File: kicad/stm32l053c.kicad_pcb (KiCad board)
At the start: 2 copper layers, 52 x 35 mm, 39 parts, among them P1 SWD, P2 PWR, Q1 BC807, Q2 BC817, SW1 SW_PUSH, SW2 SW_PUSH, SW3 SW_PUSH, SW4 SW_SPDT, U1 STM32L053C8_LQFP48, U2 TLV61225, U3 um66t, Y1 Crystal_GND23

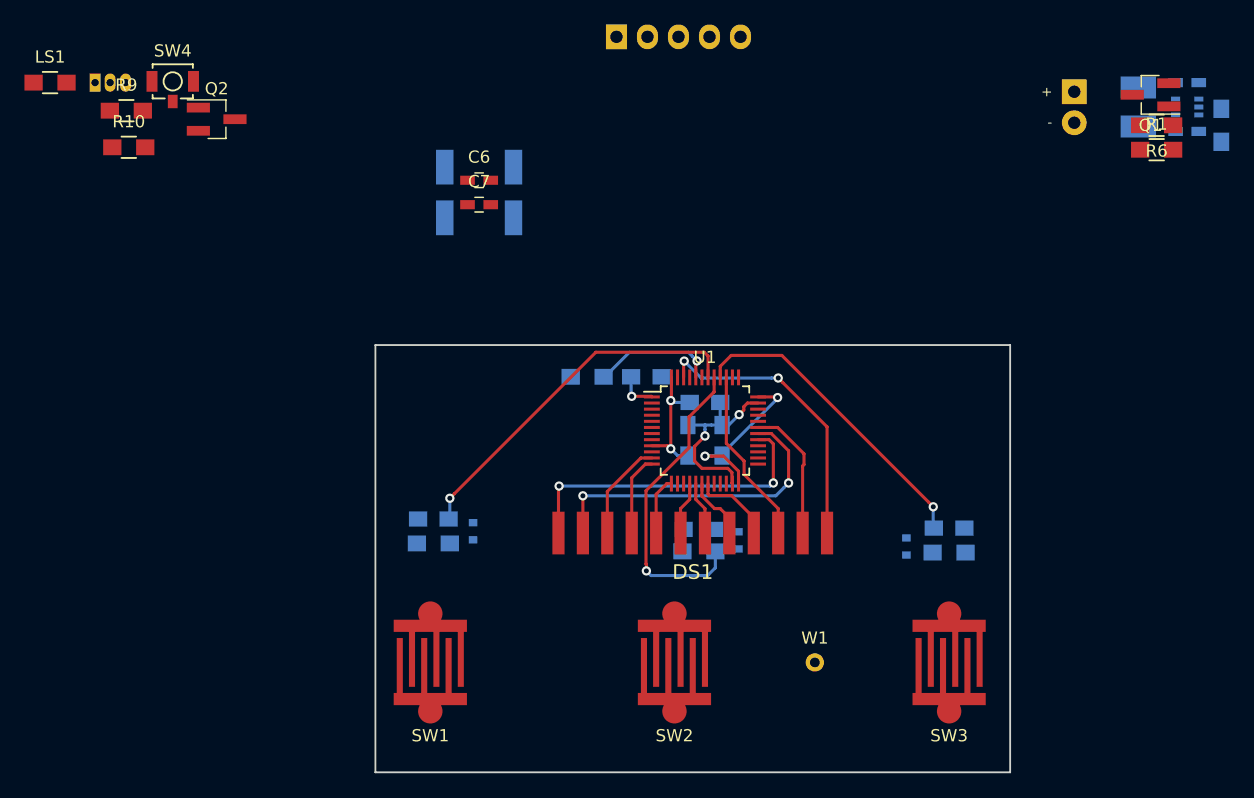
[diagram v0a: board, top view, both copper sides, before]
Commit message: Layout
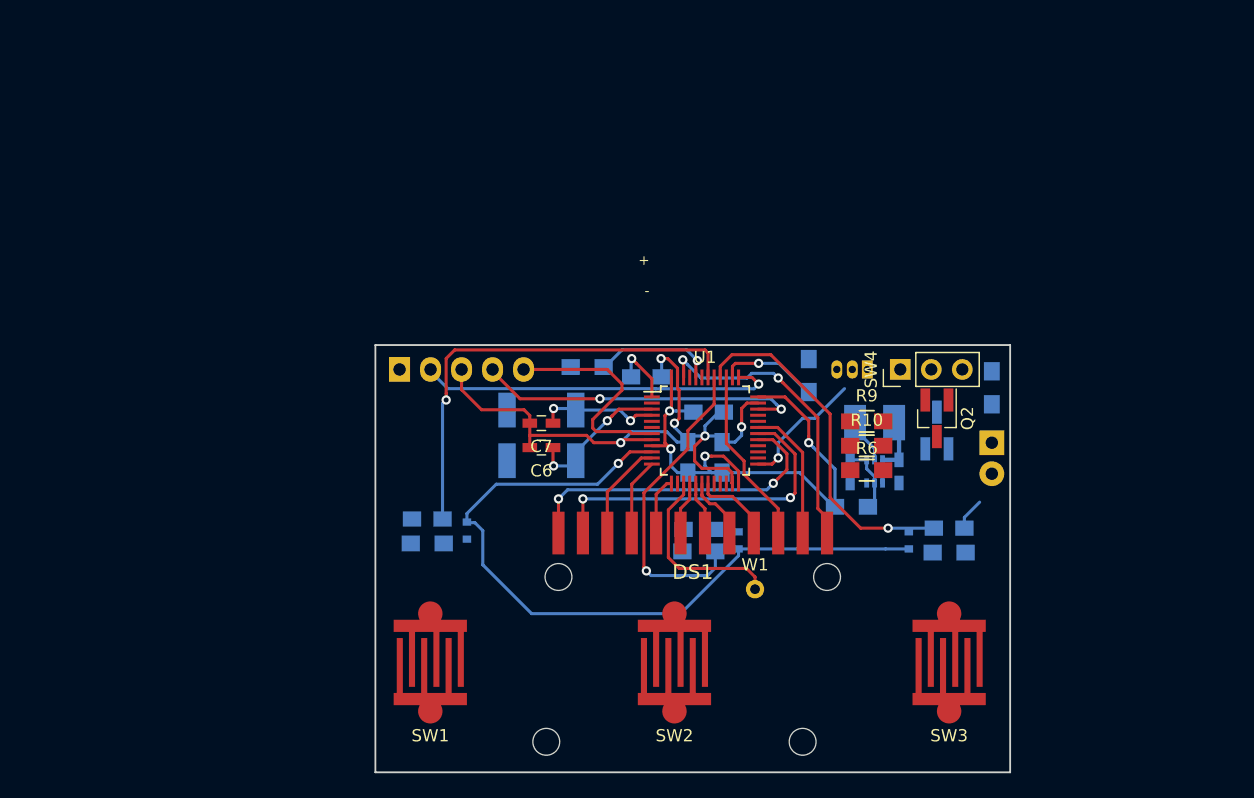
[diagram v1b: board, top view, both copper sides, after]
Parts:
- added REF**: MountingHole_2.2mm_M2, Mounting_Holes:MountingHole_2.2mm_M2, F.Cu at (131.0, 118.1)
- added REF**: MountingHole_2.2mm_M2, Mounting_Holes:MountingHole_2.2mm_M2, F.Cu at (152.0, 118.1)
- added REF**: MountingHole_2.2mm_M2, Mounting_Holes:MountingHole_2.2mm_M2, F.Cu at (154.0, 104.6)
- added REF**: MountingHole_2.2mm_M2, Mounting_Holes:MountingHole_2.2mm_M2, F.Cu at (132.0, 104.6)
- LS1, Q1, R1: moved to B.Cu
- SW4: footprint Buttons_Switches_SMD:SW_SPST_B3U-1100P -> Pin_Headers:Pin_Header_Straight_1x03_Pitch2.54mm
- moved LS1 81.1 mm to (167.5, 89.1), turned to 270 degrees
- moved R9 65.8 mm to (157.2, 91.8)
- moved R10 65.2 mm to (157.2, 93.8)
- moved SW4 64.1 mm to (160.0, 87.6), turned to 90 degrees
- moved Q2 63.9 mm to (163.0, 91.6), turned to 270 degrees
- moved U3 62.8 mm to (154.8, 87.6), turned to 0 degrees
- moved R7 43.5 mm to (156.0, 98.8), turned to 0 degrees
- moved C9 39.6 mm to (159.9, 96.0), turned to 270 degrees
- moved U2 39.3 mm to (157.9, 96.0), turned to 180 degrees
- moved C8 39.2 mm to (155.9, 96.0), turned to 270 degrees
- moved R6 36.9 mm to (157.2, 95.8), turned to 0 degrees
- moved D3 36.0 mm to (124.5, 100.8), turned to 270 degrees
- moved D1 35.7 mm to (160.7, 101.6), turned to 90 degrees
- moved R1 34.0 mm to (152.5, 88.1), turned to 270 degrees
- moved L1 33.7 mm to (157.9, 92.0), turned to 180 degrees
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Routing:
- net /WAKEUP_PIN1: track 0.00 -> 61.4 mm, vias 0 -> 1
- net Earth: track 16.2 -> 58.1 mm, vias 2 -> 5
- net SWCLK: track 0.00 -> 30.4 mm, vias 0 -> 1
- net SWDIO: track 0.00 -> 27.0 mm, vias 0 -> 2
- net VDD: track 24.7 -> 45.7 mm
- net NRST: track 0.00 -> 18.2 mm
- net Net-(U1-Pad15): track 0.00 -> 15.3 mm
- net /OSC32_IN: track 0.00 -> 11.9 mm, vias 0 -> 2
- net /MELODY: track 0.00 -> 10.4 mm, vias 0 -> 1
- net /OSC32_OUT: track 0.00 -> 9.87 mm, vias 0 -> 2
- net /BUZZER: track 0.00 -> 8.94 mm, vias 0 -> 1
- net /BUTTON2: track 29.7 -> 37.3 mm
- net +BATT: track 0.00 -> 7.04 mm
- net Net-(C8-Pad1): track 0.00 -> 5.69 mm
- net Net-(L1-Pad2): track 0.00 -> 3.71 mm
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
